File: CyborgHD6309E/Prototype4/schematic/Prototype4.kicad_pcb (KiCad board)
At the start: 2 copper layers, 95 x 72 mm, 24 parts, among them J1 Conn_AVR_UPDI, SW1 TSD1265, U1 ATmega4809-P, U2 HM628128DLP-5, U3 HD63C09E, U4 ATtiny412-SS, U5 CD74HCT30, U6 CD74HCT688

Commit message: [CyborgHD6309E] Modify Prototype4 pin maps to upcomming Prototype5
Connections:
- net /CLK_E renamed /E_CLK
- net /CLK_Q renamed /Q_CLK
- net /~USR_LED~ renamed /USR_LED
- B2 pad 2: /~DBG_RTS~ -> GND
- R2 pad 1: Net-(R2-Pad1) -> VCC
- R2 pad 2: VCC -> Net-(R2-Pad2)
- SW1 pad 1: /~USR_SW~ -> GND
- SW1 pad 2: GND -> /~USR_SW~
- SW1 pad 3: Net-(R6-Pad1) -> GND
- SW1 pad 4: VCC -> Net-(R6-Pad1)
- U1 pad 10: /~STEP~ -> /LIC
- U1 pad 11: /~INT~ -> /RD_WR
- U1 pad 16: /~RAM_E~ -> /BUSY
- U1 pad 25: /RD_WR -> /~INT~
- U1 pad 26: /~USR_SW~ -> /~STEP~
- U1 pad 28: /~DBG_RTS~ -> /~USR_SW~
- U1 pad 3: /A0 -> /~ACK~
- U1 pad 4: /A1 -> /~RAM_E~
- U1 pad 7: /~RESET~ -> /A0
- U1 pad 8: /LIC -> /A1
- U1 pad 9: /~ACK~ -> /~RESET~
- U3 pad 33: (no net) -> /BUSY
- U3 pad 4: Net-(R2-Pad1) -> Net-(R2-Pad2)

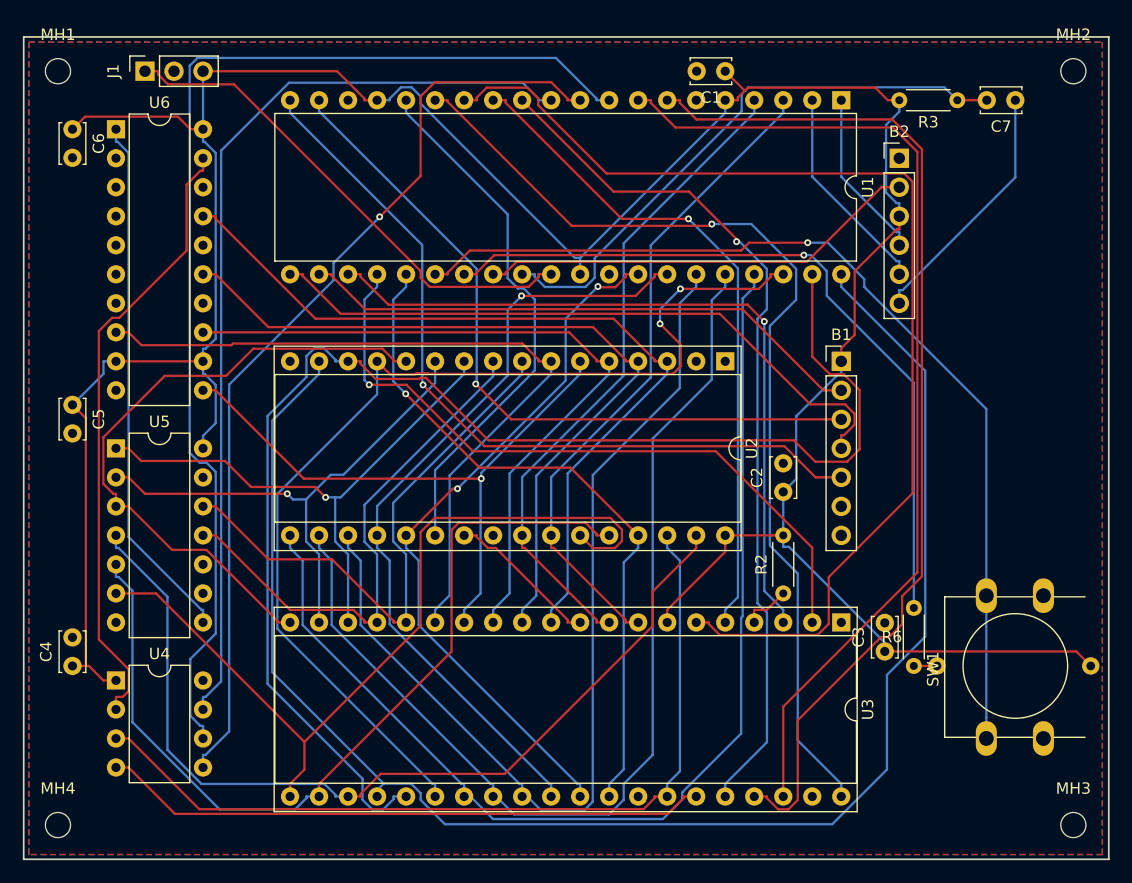
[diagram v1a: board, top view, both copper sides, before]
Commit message: [CyborgHD6309E] Prorotype5 debugger
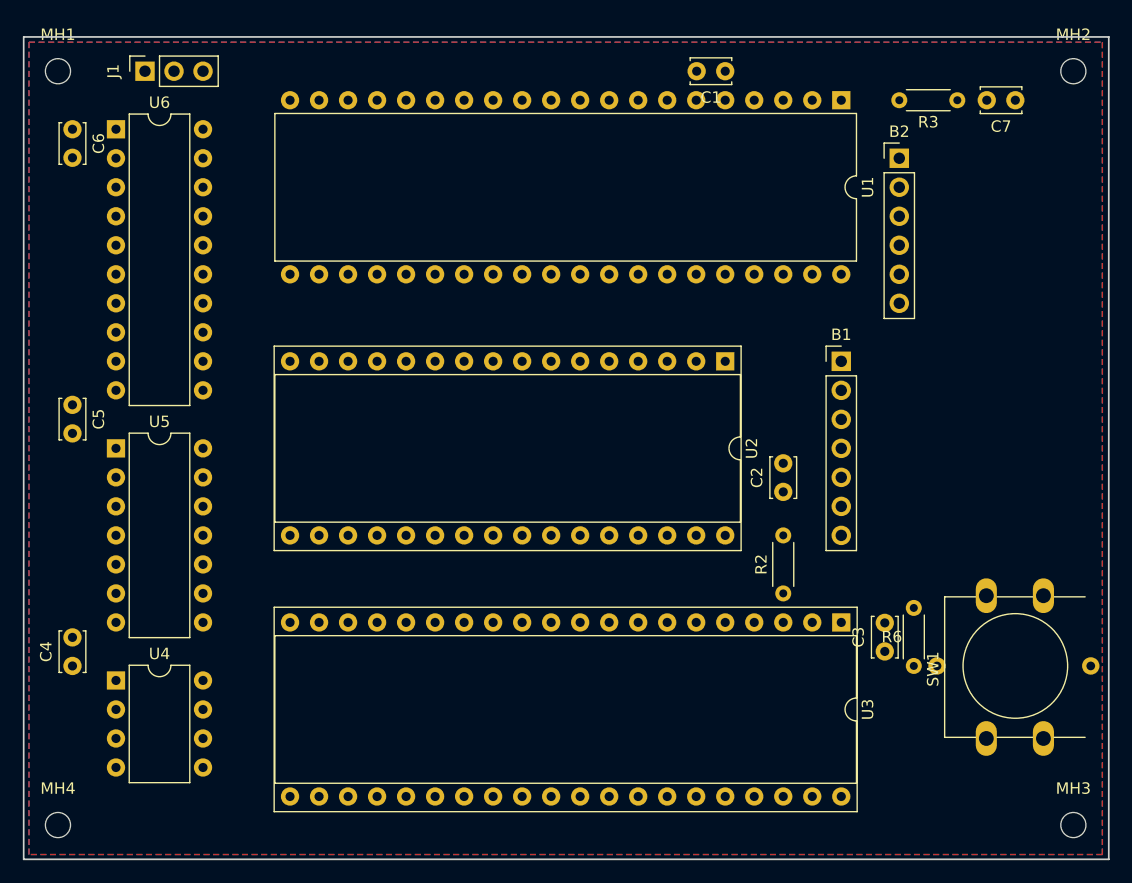
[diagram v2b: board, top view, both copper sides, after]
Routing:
- net VCC: track 260.5 -> 0.00 mm
- net /D7: track 139.7 -> 0.00 mm
- net /D6: track 119.8 -> 0.00 mm
- net /~ACK~: track 100.3 -> 0.00 mm
- net /D4: track 98.8 -> 0.00 mm
- net /BA: track 97.9 -> 0.00 mm
- net /D5: track 92.9 -> 0.00 mm, vias 2 -> 0
- net /D3: track 91.7 -> 0.00 mm
- net /~RESET~: track 90.8 -> 0.00 mm
- net /LIC: track 87.8 -> 0.00 mm
- net /~HALT~: track 87.7 -> 0.00 mm, vias 1 -> 0
- net /D2: track 86.4 -> 0.00 mm
- net /~USR_SW~: track 84.8 -> 0.00 mm, vias 1 -> 0
- net /~STEP~: track 82.0 -> 0.00 mm, vias 1 -> 0
- net /~INT~: track 81.8 -> 0.00 mm
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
